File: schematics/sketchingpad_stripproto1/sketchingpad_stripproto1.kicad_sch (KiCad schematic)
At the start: 79 parts, among them CN1 HC-1.0-4PWT, CN2 S2B-PH-SM4-TB, J3 AudioJack4, Q1 AO3415A, SW1 TS-1088-AR02016, U1 TS20, U2 Seeeduino Xiao nRF52840

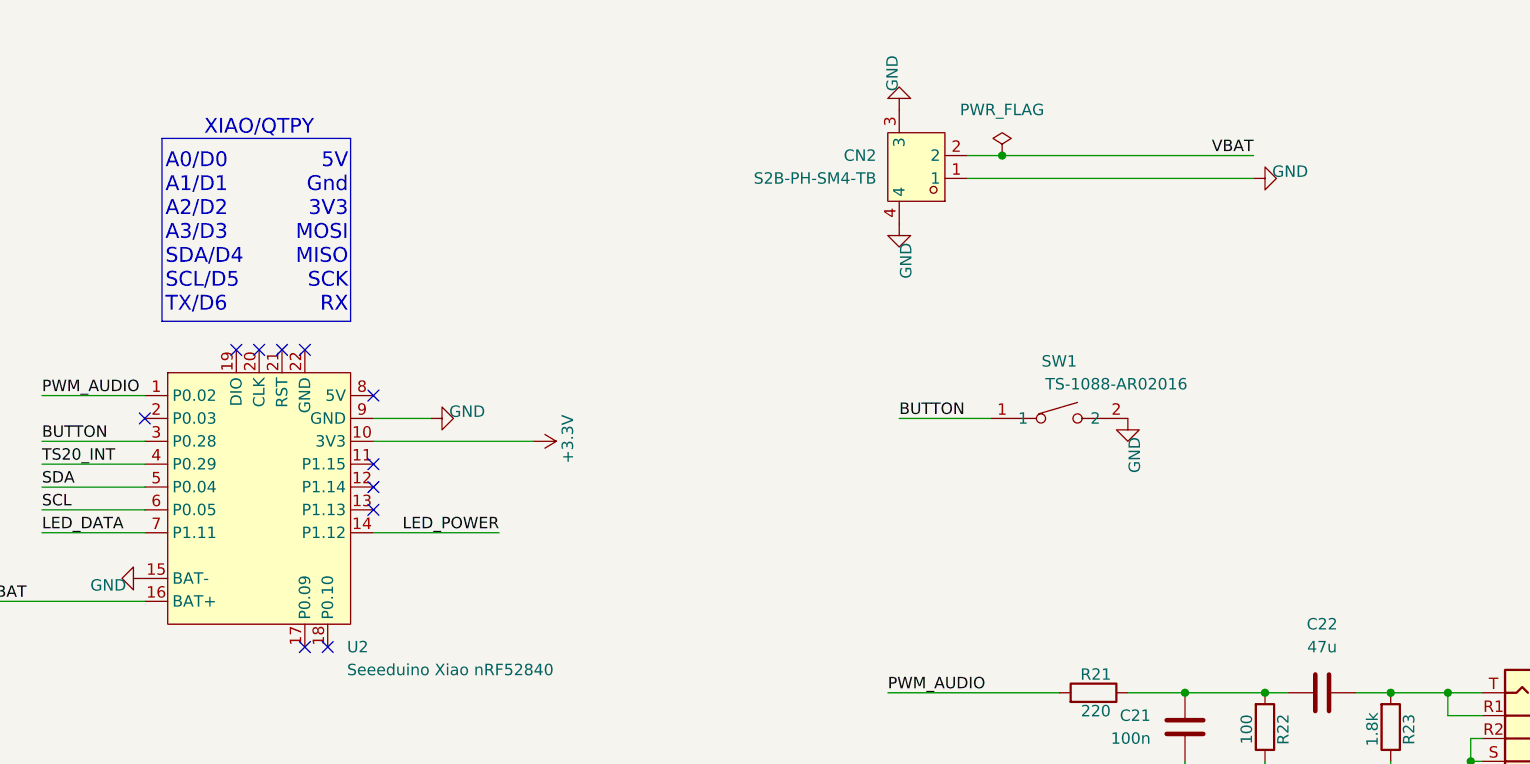
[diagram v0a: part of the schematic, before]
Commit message: final on the sketchingpad_stripproto1 sch maybe
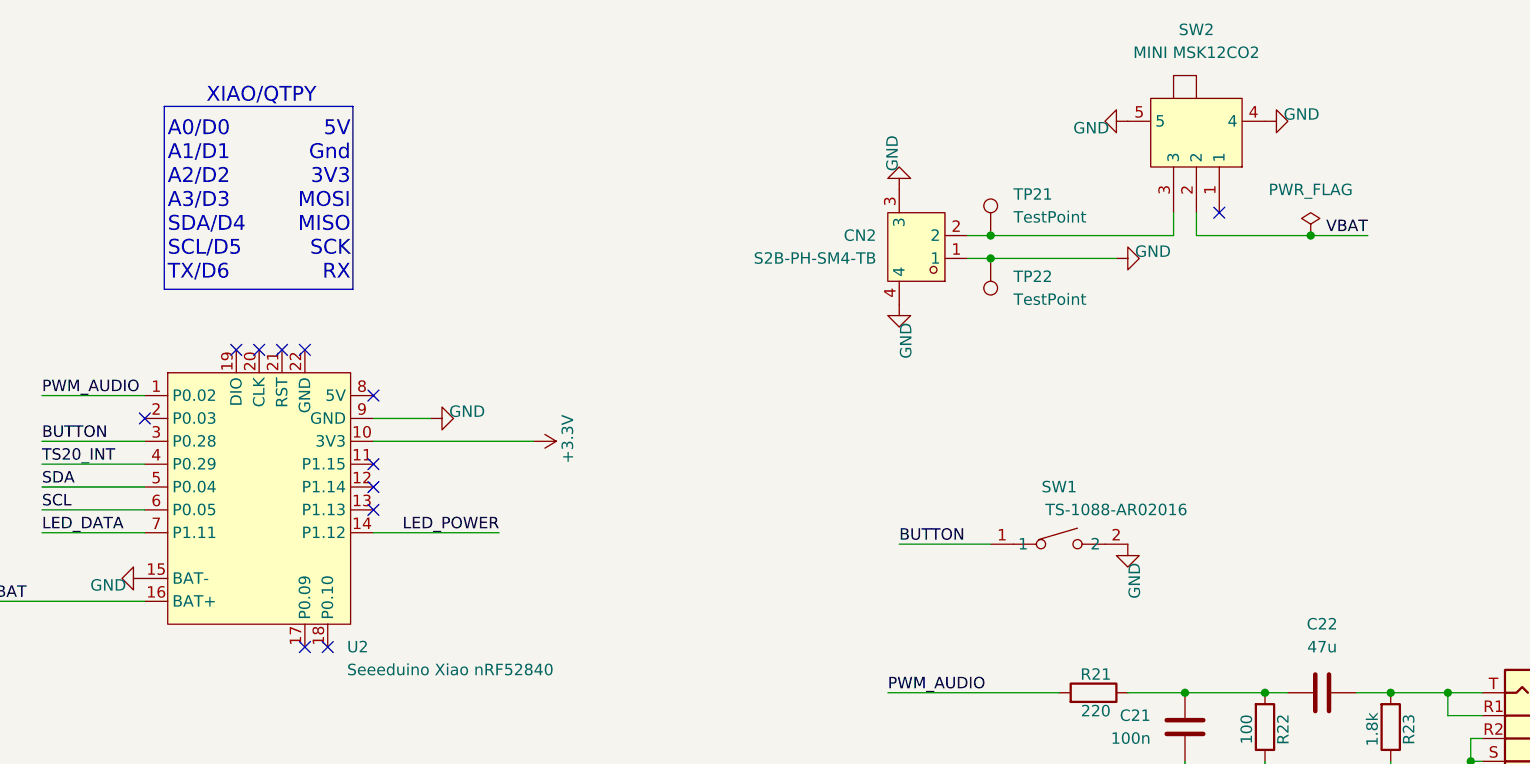
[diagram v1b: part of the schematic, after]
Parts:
- added SW2: MINI MSK12CO2, easyeda2kicad:SW-SMD_MSK12CO2, symbol easyeda2kicad:MINIMSK12CO2
- added TP21, TP22: TestPoint, TestPoint:TestPoint_Pad_D1.5mm, symbol Connector:TestPoint
- U2: footprint PCM_marbastlib-xp-promicroish:Xiao_nRF52840_ACH -> todbot_stuff:Xiao_nRF52840_ACH-todedit
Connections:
- net GND: now also SW2.4, SW2.5, TP22.1
- net VBAT: now also SW2.2; no longer CN2.2
- new net: CN2.2, SW2.3, TP21.1
- no-connect marks 12 -> 13
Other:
- moved on the sheet: CN2, SW1
